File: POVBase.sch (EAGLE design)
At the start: 19 parts, among them IC1 LM2576S, Q5 IRF540, Q6 IRF540

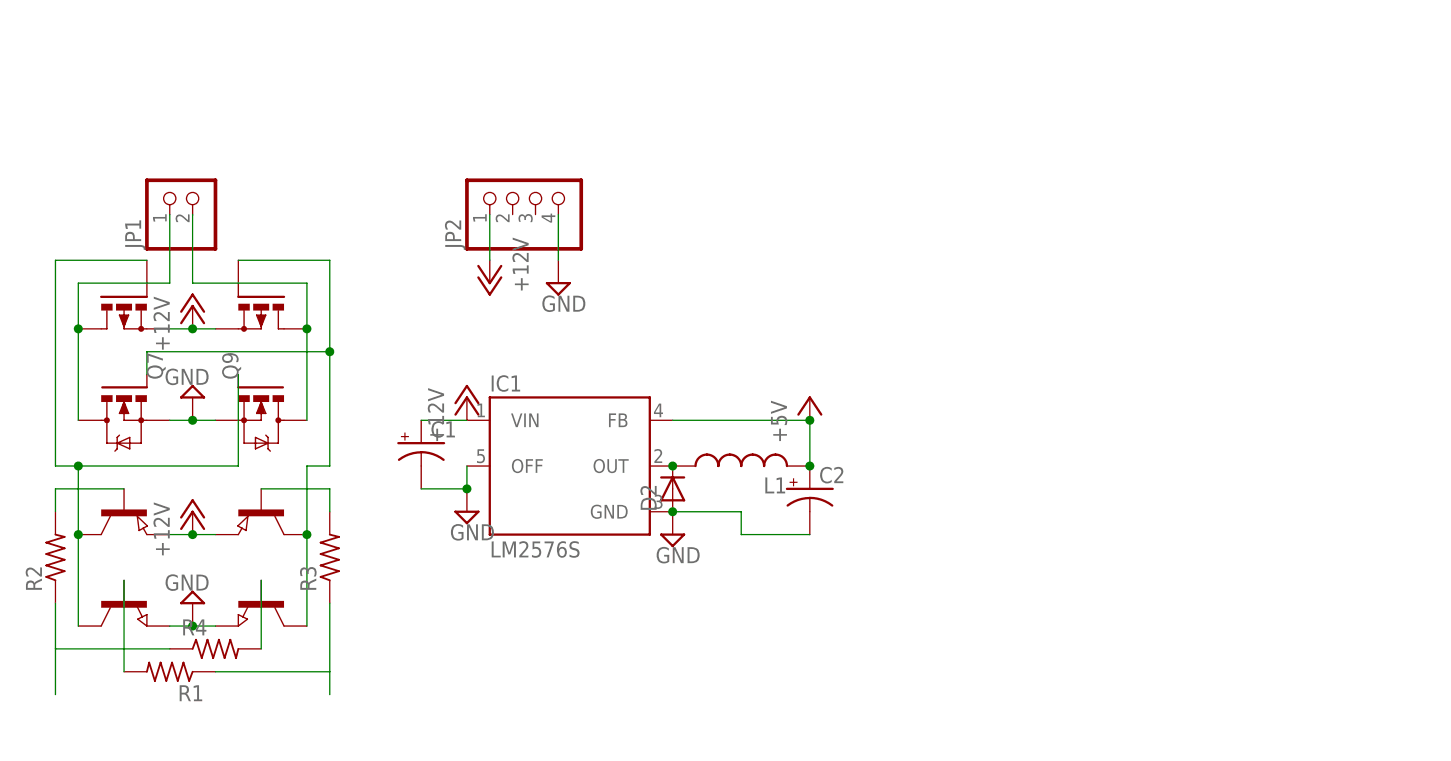
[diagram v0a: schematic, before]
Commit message: xgns
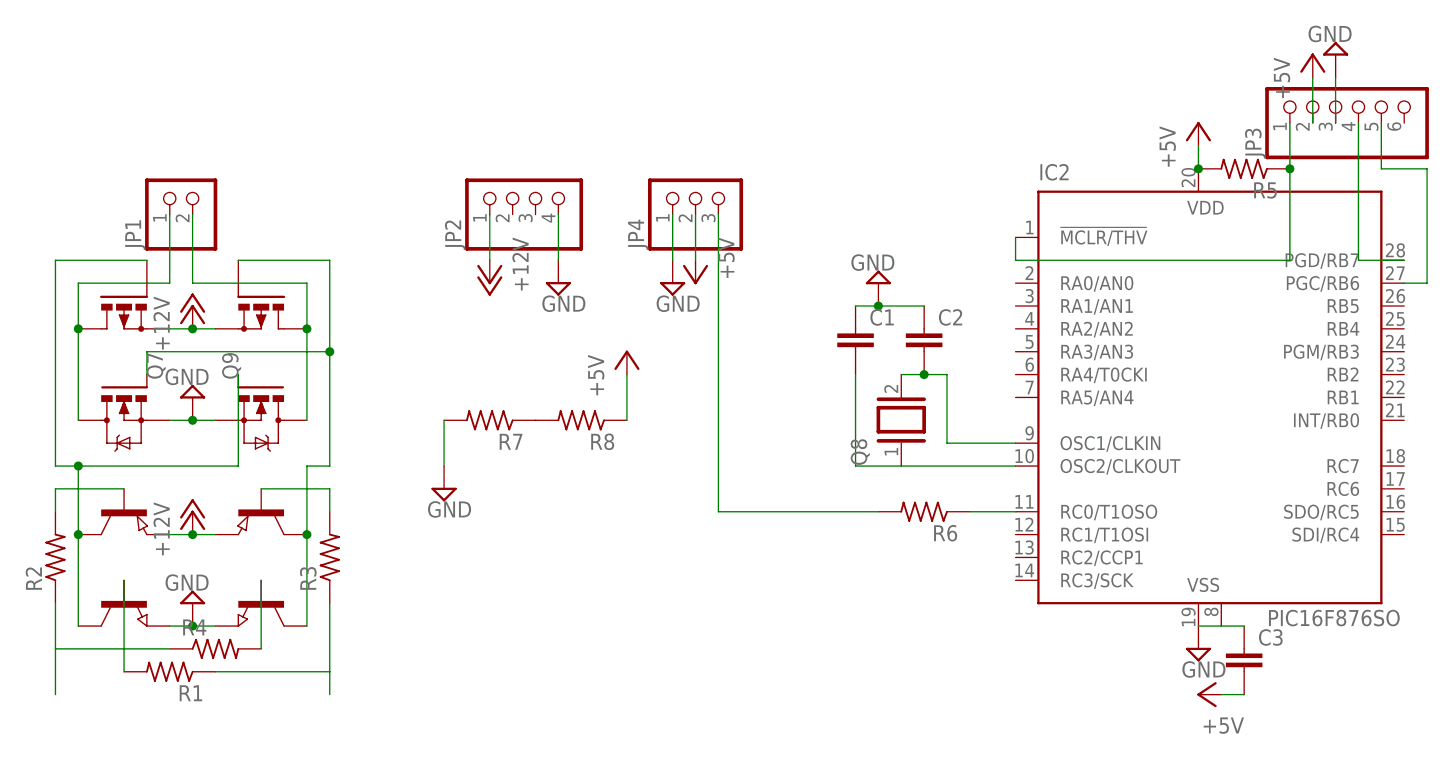
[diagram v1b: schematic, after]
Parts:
- removed D2: (no value), semicon-smd-ipc:D-MLL-41
- removed IC1: LM2576S, lm2576:LM2576S
- removed L1: (no value), rcl:L-US6000-XXX-RC
- added C3: (no value), resistor:C-EUC0805
- added IC2: PIC16F876SO, microchip:PIC16F876SO
- added JP3: (no value), pinhead:PINHD-1X6
- added JP4: (no value), pinhead:PINHD-1X3
- added Q8: (no value), special:XTAL/S
- added R5, R6, R7, R8: (no value), resistor:R-US_R0805
- C1: device rcl:CPOL-USCT7343 -> resistor:C-EUC0805
- C2: device rcl:CPOL-US153CLV-1014 -> resistor:C-EUC0805
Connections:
- new net N$12: IC2.!MCLR/THV, JP3.1, R5.1
- new net N$13: IC2.PGD/RB7, JP3.4
- new net N$14: IC2.PGC/RB6, JP3.5
- new net N$15: IC2.RC0/T1OSO, R6.1
- new net N$16: C1.2, IC2.OSC2/CLKOUT, Q8.1
- new net N$17: C2.2, IC2.OSC1/CLKIN, Q8.2
- new net N$20: R7.1, R8.2
- net +12V: no longer C1.+, IC1.VIN
- net +5V: now also C3.2, IC2.VDD, JP3.2, JP4.2, R5.2, R8.1; no longer C2.+, IC1.FB, L1.2
- net GND: now also C1.1, C2.1, C3.1, IC2.VSS, IC2.VSS@1, JP3.3, JP4.1, R7.2; no longer C1.-, C2.-, D2.A, IC1.GND, IC1.OFF
- net N$9: now also JP4.3, R6.2; no longer D2.C, IC1.OUT, L1.1
